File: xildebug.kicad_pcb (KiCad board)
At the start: 2 copper layers, 42 x 46.2 mm, 66 parts, among them J1 USB_B_Micro, J2 Conn_STM_SWD, J3 Conn_Ext1, J4 Conn_Ext2, J5 Conn_DUT, J6 Conn_DUT_VDD, SW1 BOOT0, U1 XC6206P332MR, U2 MAX14662, U3 STM32L433CCUx, U4 TS5A3167, U5 MIC5219YMT, U6 TS5A3167, U7 MCP4018, U8 TS5A3167

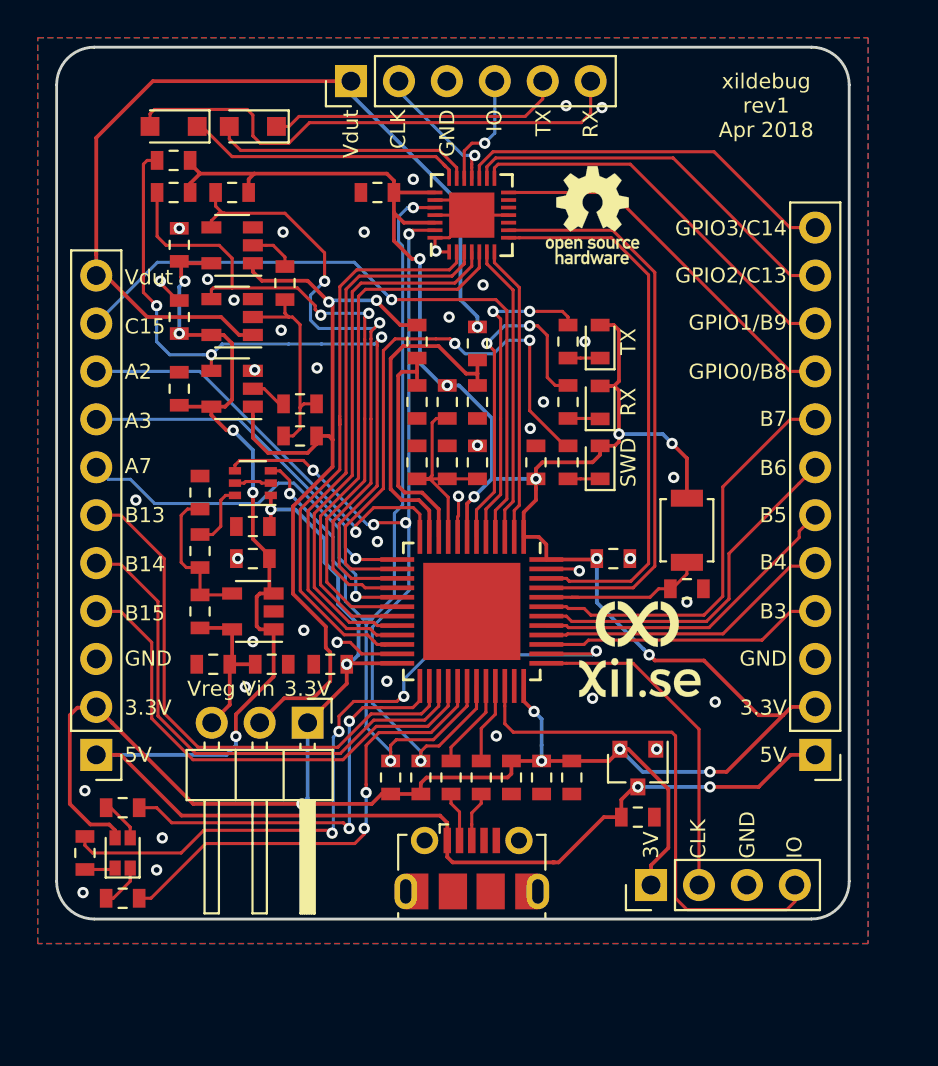
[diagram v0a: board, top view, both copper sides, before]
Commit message: Minification
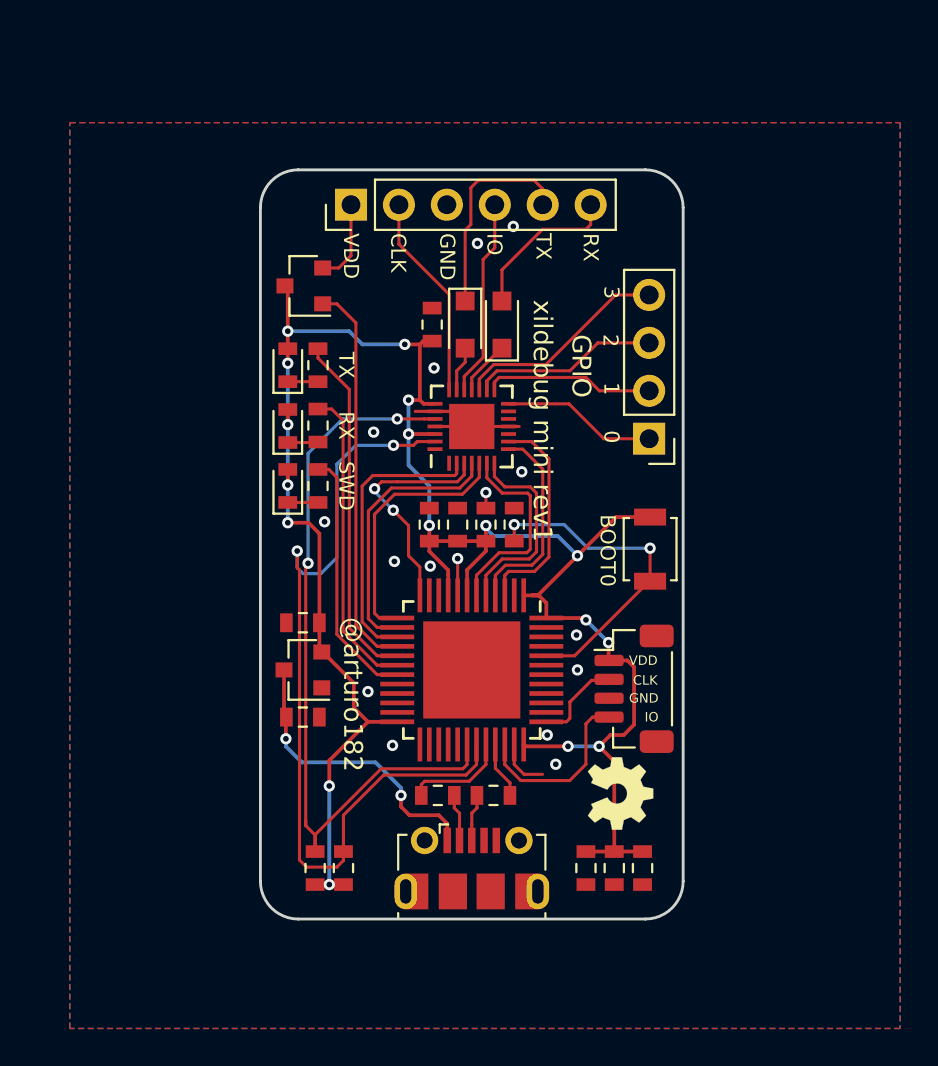
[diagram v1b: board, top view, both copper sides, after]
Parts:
- removed C11, C15: 1uF, Capacitor_SMD:C_0603_1608Metric
- removed C12, C14, C17, C18, C19, C8: 0.1uF, Capacitor_SMD:C_0603_1608Metric
- removed C13: 4.7uF, Capacitor_SMD:C_0603_1608Metric
- removed C16: 470pF, Capacitor_SMD:C_0603_1608Metric
- removed D4: LED_RGB, LED_SMD_Extra:LED_RGB_0606_1616Metric
- removed the G*** at (228.9, 85.4)
- removed the G*** at (226.4, 62.4)
- removed J4: Conn_Ext2, Connector_PinHeader_2.54mm:PinHeader_1x12_P2.54mm_Vertical
- removed J6: Conn_DUT_VDD, Connector_PinHeader_2.54mm:PinHeader_1x03_P2.54mm_Horizontal
- removed L1: FB, Inductor_SMD:L_0603_1608Metric
- removed R11, R15, R17: 10K, Resistor_SMD:R_0603_1608Metric
- removed R12, R14: TBD, Resistor_SMD:R_0603_1608Metric
- removed R13: 510R, Resistor_SMD:R_0603_1608Metric
- removed R16: 33R, Resistor_SMD:R_0603_1608Metric
- removed R18: 1.8R, Resistor_SMD:R_0603_1608Metric
- removed R19, R20, R21, R22: 100K, Resistor_SMD:R_0603_1608Metric
- removed R4, R5, R6: 360R, Resistor_SMD:R_0603_1608Metric
- removed U4, U6, U8: TS5A3167, Package_TO_SOT_SMD:SOT-23-5
- removed U5: MIC5219YMT, Package_TO_SOT_SMD:SOT-23-5
- removed U7: MCP4018, Package_TO_SOT_SMD:SOT-363_SC-70-6
- added G***: LOGO, Symbol_Extra:xil_5000, B.Cu at (220.0, 86.7)
- added G***: LOGO, Symbol_Extra:oshw_crop_10000, F.Cu at (227.8, 93.0)
- added Q1: FDN340P, Package_TO_SOT_SMD:SOT-23, F.Cu at (211.1, 66.2)
- J2: footprint Connector_PinHeader_2.54mm:PinHeader_1x04_P2.54mm_Vertical -> Connector_JST:JST_SH_BM04B-SRSS-TB_1x04-1MP_P1.00mm_Vertical
- J3: value Conn_Ext1 -> Conn_GPIO; footprint Connector_PinHeader_2.54mm:PinHeader_1x11_P2.54mm_Vertical -> Connector_PinHeader_2.54mm:PinHeader_1x04_P2.54mm_Vertical
- moved J3 33.7 mm to (229.4, 74.2)
- moved D6 18.7 mm to (219.7, 68.2), turned to 270 degrees
- moved C9 18.5 mm to (211.1, 89.0)
- moved U1 18.5 mm to (211.1, 86.5), turned to 180 degrees
- moved D5 16.9 mm to (221.6, 68.2), turned to 90 degrees
- moved D1 16.6 mm to (210.2, 76.8)
- moved D2 16.6 mm to (210.2, 70.3)
- moved D3 16.6 mm to (210.2, 73.6)
- moved R1 13.3 mm to (211.8, 76.8)
- moved R2 13.3 mm to (211.8, 70.3)
- moved R3 13.3 mm to (211.8, 73.5)
- moved U2 11.2 mm to (220.0, 73.6)
- moved J2 10.4 mm to (228.6, 87.5), turned to 270 degrees
- moved R23 9.76 mm to (222.2, 78.8), turned to 90 degrees
- moved C3 7.58 mm to (217.9, 68.2), turned to 90 degrees
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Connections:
- net /POT_SCL renamed /STM_SCL
- net /POT_SDA renamed /STM_SDA
- C7 pad 1: Net-(C11-Pad1) -> +3V3
- D5 pad 1: /DUT_UART_TX_B -> Net-(D5-Pad1)
- D5 pad 2: Net-(D5-Pad2) -> /DUT_UART_RX_B
- D6 pad 1: Net-(D6-Pad1) -> /DUT_UART_TX_B
- D6 pad 2: /DUT_UART_RX_B -> Net-(D6-Pad2)
- J3 pad 1: +5V -> /GPIO0_B
- J3 pad 2: +3V3 -> /GPIO1_B
- J3 pad 3: GND -> /GPIO2_B
- J3 pad 4: /PB15 -> /GPIO3_B
- J5 pad 1: /DUT_VDD_OUT -> Net-(J5-Pad1)
- U2 pad 18: /DUT_SWCLK_B -> Net-(D5-Pad1)
- U2 pad 2: /DUT_UART_RX_A -> /DUT_SWCLK_A
- U2 pad 20: Net-(D5-Pad2) -> Net-(D6-Pad2)
- U2 pad 21: Net-(D6-Pad1) -> /DUT_SWCLK_B
- U2 pad 5: /DUT_SWCLK_A -> /DUT_UART_RX_A
- U3 pad 10: /DUT_VDD_IN_DIV -> Net-(U3-Pad10)
- U3 pad 11: /DUT_VDD_OUT_DIV -> Net-(U3-Pad11)
- U3 pad 12: /PA2 -> /DUT_UART_TX_A
- U3 pad 13: /PA3 -> /DUT_UART_RX_A
- U3 pad 14: /DUT_SWD_LED -> /DUT_SWDIO_A
- U3 pad 15: /SHUNT1_EN -> /DUT_SWCLK_A
- U3 pad 16: /SHUNT2_EN -> /DUT_VDD_CTRL
- U3 pad 17: /PA7 -> /DUT_UART_TX_LED
- U3 pad 18: /DUT_VDD_EN -> /DUT_UART_RX_LED
- U3 pad 19: /DUT_SWCLK_A -> /DUT_SWD_LED
- U3 pad 2: /GPIO2_A -> Net-(U3-Pad2)
- U3 pad 20: /DUT_SWDIO_A -> Net-(U3-Pad20)
- U3 pad 21: /DUT_UART_TX_A -> Net-(U3-Pad21)
- U3 pad 22: /DUT_UART_RX_A -> Net-(U3-Pad22)
- U3 pad 25: /LED_RGB_B -> Net-(U3-Pad25)
- U3 pad 26: /PB13 -> Net-(U3-Pad26)
- U3 pad 27: /PB14 -> Net-(U3-Pad27)
- U3 pad 28: /PB15 -> Net-(U3-Pad28)
- U3 pad 29: /LED_RGB_G -> Net-(U3-Pad29)
- U3 pad 3: /GPIO3_A -> /GPIO0_A
- U3 pad 38: /LED_RGB_R -> Net-(U3-Pad38)
- U3 pad 39: /PB3 -> Net-(U3-Pad39)
- U3 pad 4: /PC15 -> /GPIO1_A
- U3 pad 40: /PB4 -> Net-(U3-Pad40)
- U3 pad 41: /PB5 -> Net-(U3-Pad41)
- U3 pad 42: /PB6 -> Net-(U3-Pad42)
- U3 pad 43: /PB7 -> Net-(U3-Pad43)
- U3 pad 45: /GPIO0_A -> Net-(U3-Pad45)
- U3 pad 46: /GPIO1_A -> Net-(U3-Pad46)
- U3 pad 5: /DUT_UART_TX_LED -> /GPIO2_A
- U3 pad 6: /DUT_UART_RX_LED -> /GPIO3_A
- U3 pad 9: Net-(C11-Pad1) -> +3V3
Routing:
- net +5V: track 88.7 -> 15.8 mm, vias 7 -> 2
- net +3V3: track 176.9 -> 112.3 mm, vias 15 -> 17
- net /DUT_VDD_OUT: track 48.1 -> 0.00 mm, vias 1 -> 0
- net /DUT_VDD_IN: track 43.6 -> 0.00 mm, vias 2 -> 0
- net /SHUNT1_EN: track 40.4 -> 0.00 mm, vias 3 -> 0
- net /LED_RGB_R: track 39.0 -> 0.00 mm, vias 4 -> 0
- net /DUT_VDD_EN: track 37.5 -> 0.00 mm, vias 2 -> 0
- net /PC15: track 36.4 -> 0.00 mm, vias 1 -> 0
- net /SHUNT2_EN: track 34.5 -> 0.00 mm, vias 2 -> 0
- net /PB13: track 29.5 -> 0.00 mm
- net /PB14: track 28.0 -> 0.00 mm
- net /PB15: track 26.5 -> 0.00 mm
- net /LED_RGB_G: track 24.9 -> 0.00 mm, vias 2 -> 0
- net /PA2: track 22.9 -> 0.00 mm, vias 1 -> 0
- net /LED_RGB_B: track 22.2 -> 0.00 mm, vias 2 -> 0
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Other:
- board size 42 x 46.2 mm -> 22.4 x 39.7 mm
- board text added: "0"
- board text added: "1"
- board text added: "2"
- board text added: "3"
- board text added: "@arturo182"
- board text added: "BOOT0"
- board text added: "GPIO"
- board text added: "VDD"
- board text added: "xildebug mini rev1"
- board text removed: "3.3V"
- board text removed: "3V"
- board text removed: "5V"
- board text removed: "A2"
- board text removed: "A3"
- board text removed: "A7"
- board text removed: "B13"
- board text removed: "B14"
- board text removed: "B15"
- board text removed: "B3"
- board text removed: "B4"
- board text removed: "B5"
- board text removed: "B6"
- board text removed: "B7"
- board text removed: "C15"
- board text removed: "GPIO0/B8"
- board text removed: "GPIO1/B9"
- board text removed: "GPIO2/C13"
- board text removed: "GPIO3/C14"
- board text removed: "Vdut"
- board text removed: "Vin"
- board text removed: "Vreg"
- board text removed: "xildebug rev1 Apr 2018"
